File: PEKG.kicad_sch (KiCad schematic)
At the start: 115 parts, among them J1 AudioJack4, J2 AudioJack3_SwitchTR, U1 TLV9062, U12 NCS21802DMR2G, U13 NCS21802DMR2G, U2 TLV9062, U3 INA350CDSIDDFR, U7 TLV61070ADBVR, U8 NCS21802DMR2G

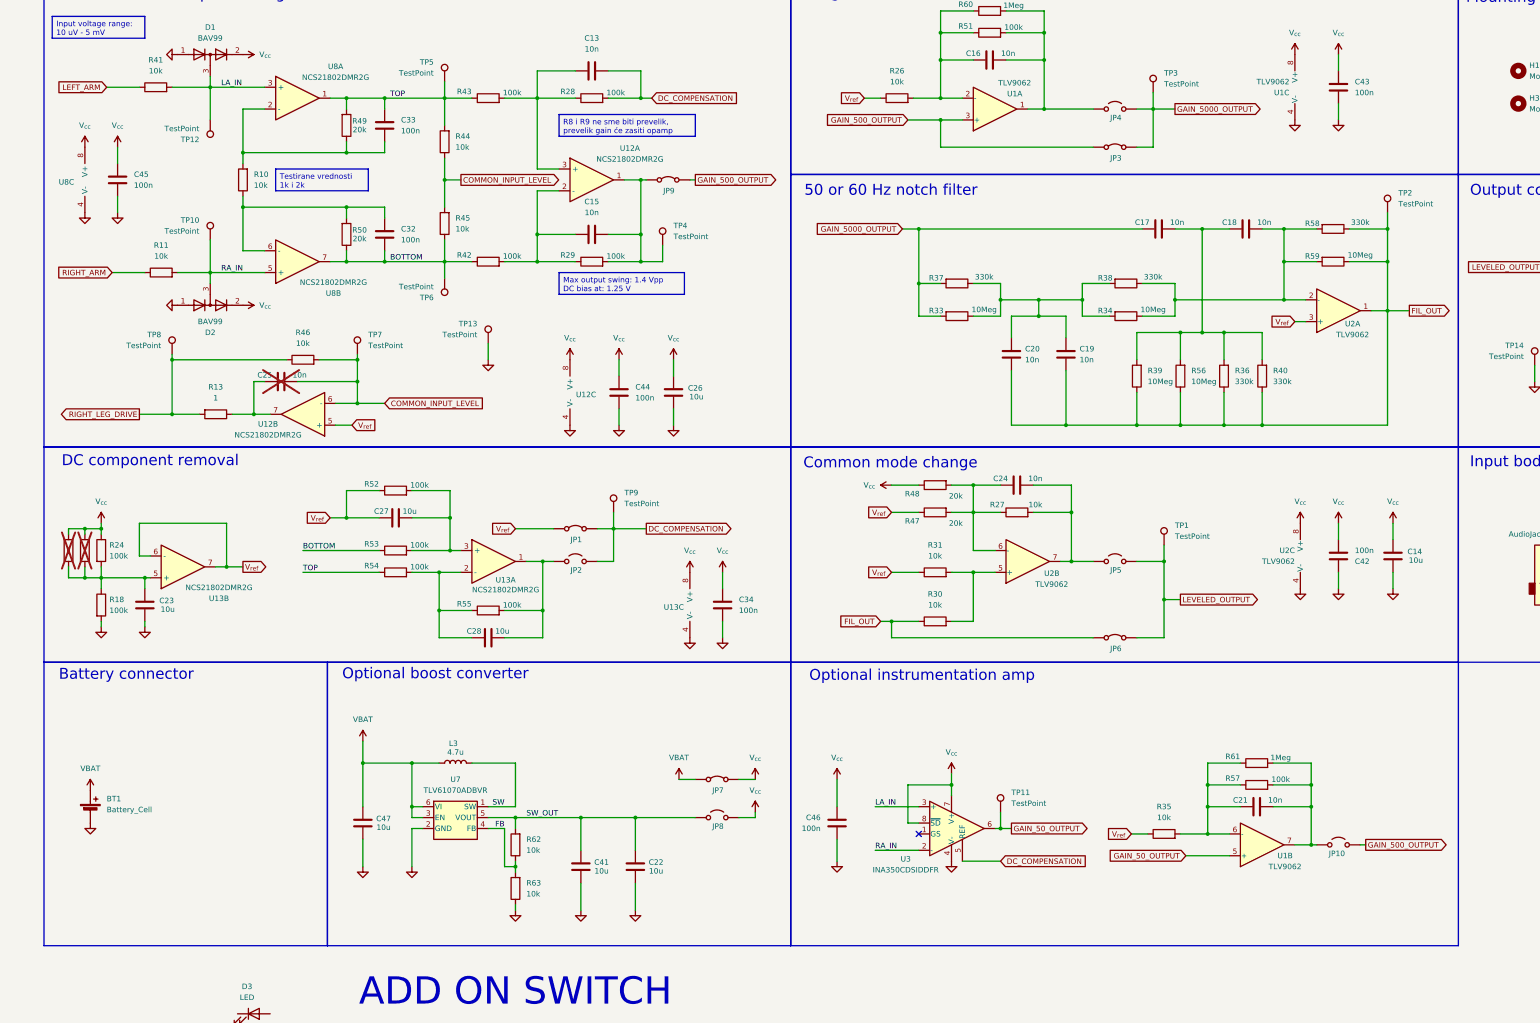
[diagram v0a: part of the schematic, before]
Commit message: added sw
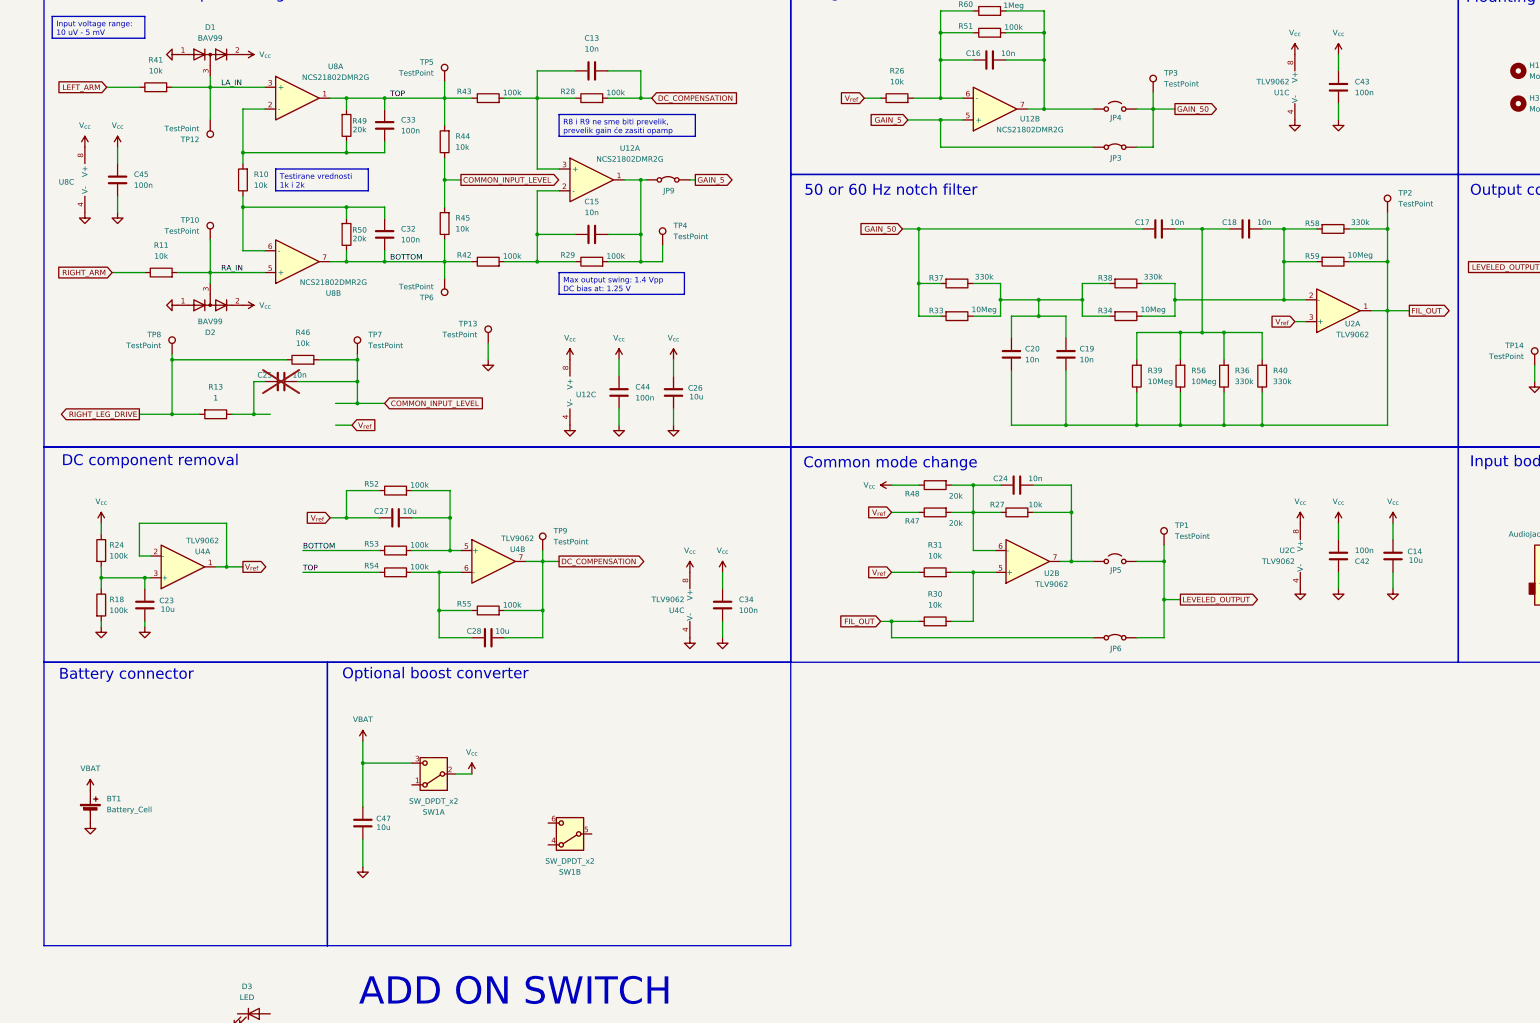
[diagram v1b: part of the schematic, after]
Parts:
- removed C21: 10n, Capacitor_SMD:C_0603_1608Metric_Pad1.08x0.95mm_HandSolder, symbol Device:C
- removed C22, C41: 10u, Capacitor_SMD:C_0603_1608Metric_Pad1.08x0.95mm_HandSolder, symbol Device:C
- removed C46: 100n, Capacitor_SMD:C_0603_1608Metric_Pad1.08x0.95mm_HandSolder, symbol Device:C
- removed JP1, JP7: Jumper_2_Bridged, Jumper:SolderJumper-2_P1.3mm_Bridged_RoundedPad1.0x1.5mm, symbol Jumper:Jumper_2_Bridged
- removed JP10, JP2, JP8: Jumper_2_Open, Jumper:SolderJumper-2_P1.3mm_Open_RoundedPad1.0x1.5mm, symbol Jumper:Jumper_2_Open
- removed L3: 4.7u, Inductor_SMD:L_Bourns_SRN6045TA, symbol Device:L
- removed R23, R32, R57: 100k, Resistor_SMD:R_0603_1608Metric_Pad0.98x0.95mm_HandSolder, symbol Device:R
- removed R35, R62, R63: 10k, Resistor_SMD:R_0603_1608Metric_Pad0.98x0.95mm_HandSolder, symbol Device:R
- removed R61: 1Meg, Resistor_SMD:R_0603_1608Metric_Pad0.98x0.95mm_HandSolder, symbol Device:R
- removed TP11: TestPoint, TestPoint:TestPoint_Pad_D3.0mm, symbol Connector:TestPoint
- removed unit 2 of U1
- removed unit 1 of U1
- removed U13: NCS21802DMR2G, Package_SO:OnSemi_Micro8, symbol voltmeter_lib:NCS21802DMR2G
- removed U3: INA350CDSIDDFR, Package_SO:MSOP-8_3x3mm_P0.65mm, symbol PEKG_lib:INA350CDSIDDFR
- removed U7: TLV61070ADBVR, Package_TO_SOT_SMD:SOT-23-6_Handsoldering, symbol DS100M08KV:TLV61070ADBVR
- added SW1: SW_DPDT_x2, PEKG:DPDT_bigger, symbol Switch:SW_DPDT_x2
- added U4: TLV9062, Package_SO:SOIC-8_3.9x4.9mm_P1.27mm, symbol Amplifier_Operational:TLV9062
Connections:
- net COMMON_INPUT_LEVEL: no longer U12.6 (-)
- net DC_COMPENSATION: now also C28.2, R55.2, U4.7
- net GND: now also U4.4 (V-)
- net VBAT: now also SW1.3 (C)
- net V_{cc}: now also SW1.2 (B), U4.8 (V+)
- net V_{ref}: now also U4.1, U4.2 (-); no longer U12.5 (+)
- net at C27.2, R52.2, R53.2: now also U4.5 (+)
- net at C23.1, R18.1, R24.2: now also U4.3 (+)
- net at C16.2, R26.2, R51.1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: now also U12.6 (-)
- net at C16.1, JP4.1 (A), R51.2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: now also U12.7
- net at C25.2, R13.1: no longer U12.7
- net at C28.1, R54.2, R55.1: now also U4.6 (-)
- net GAIN_5000_OUTPUT renamed GAIN_50
- net GAIN_500_OUTPUT renamed GAIN_5
- net GAIN_5: now also U12.5 (+)
- no-connect marks 5 -> 4
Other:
- note removed: "Optional instrumentation amp"
- moved on the sheet: TP9

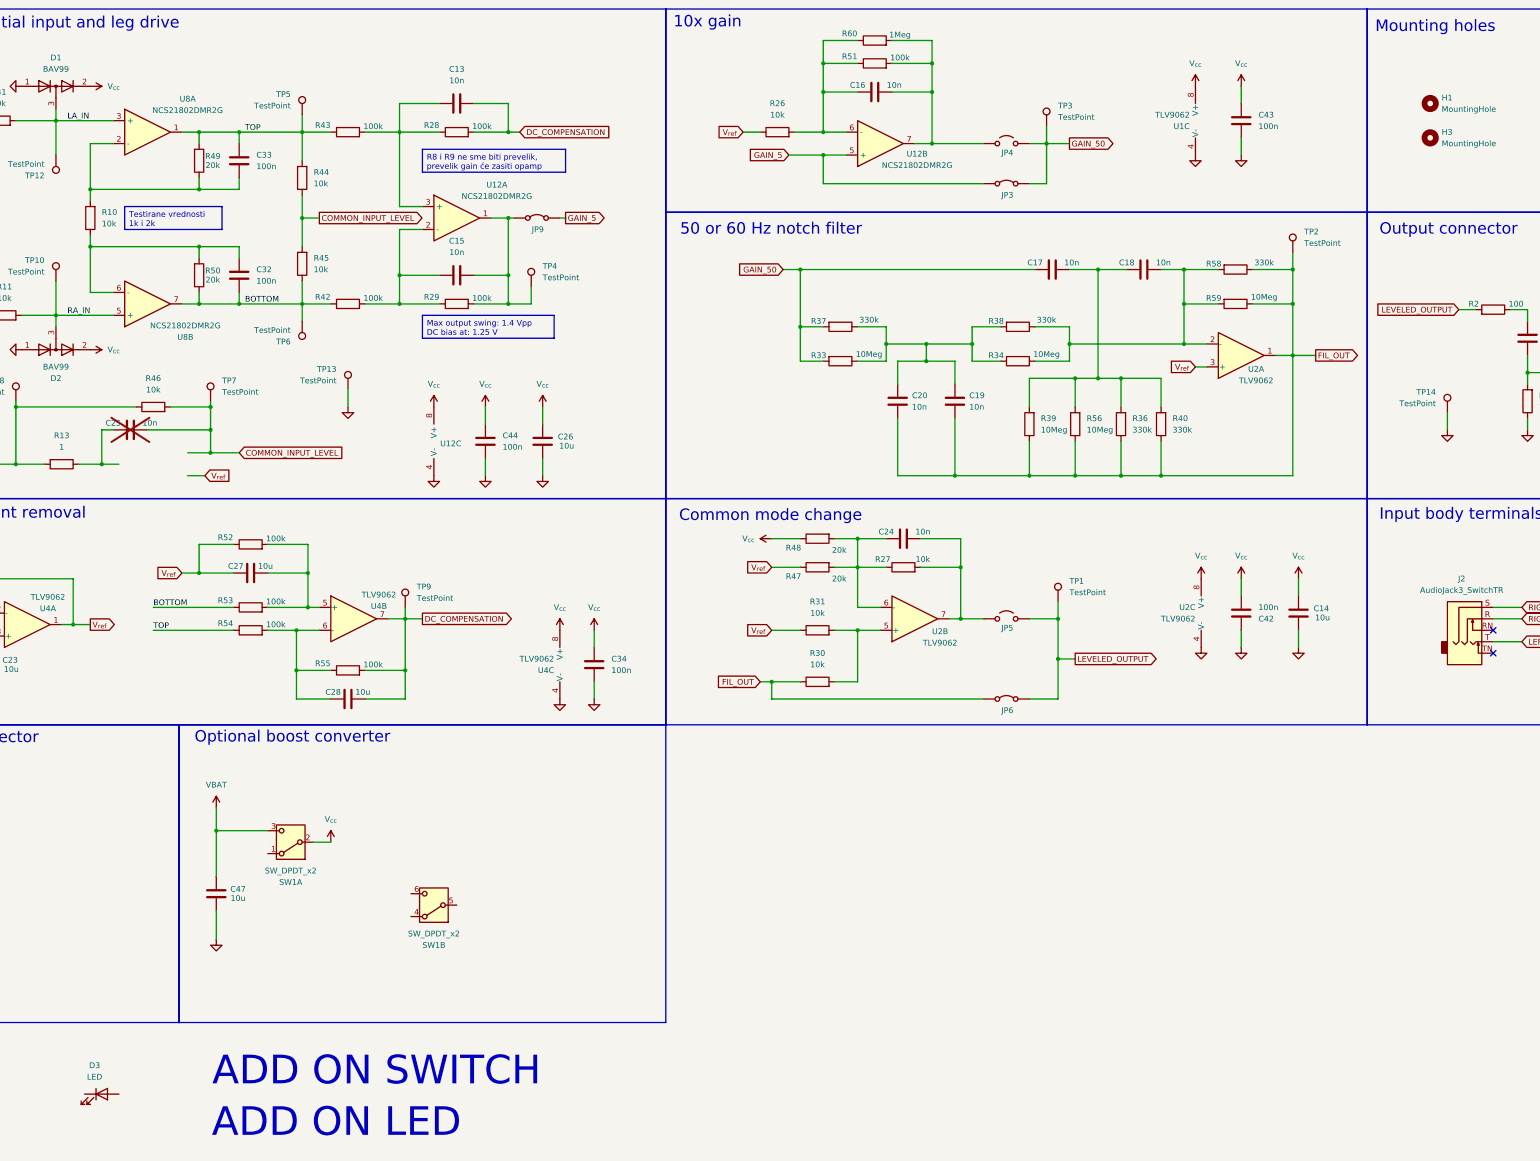
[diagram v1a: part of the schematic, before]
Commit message: opop
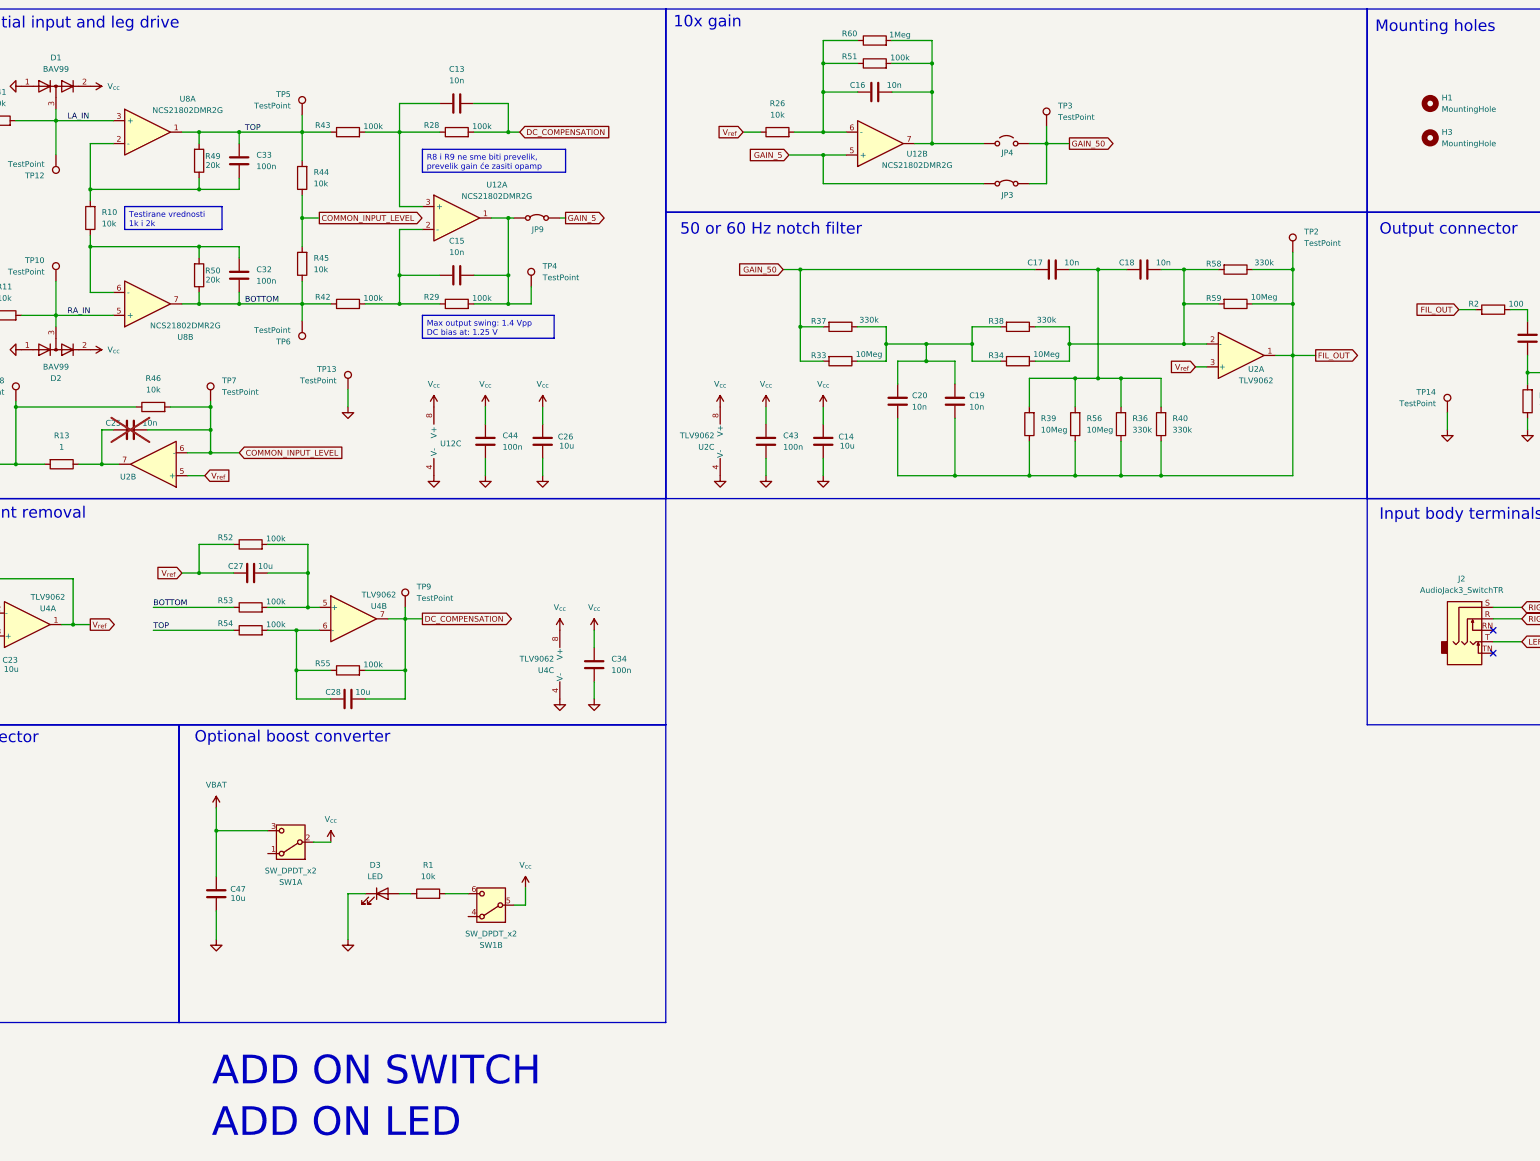
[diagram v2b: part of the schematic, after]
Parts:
- removed C24: 10n, Capacitor_SMD:C_0603_1608Metric_Pad1.08x0.95mm_HandSolder, symbol Device:C
- removed C42: 100n, Capacitor_SMD:C_0603_1608Metric_Pad1.08x0.95mm_HandSolder, symbol Device:C
- removed JP5: Jumper_2_Open, Jumper:SolderJumper-2_P1.3mm_Open_RoundedPad1.0x1.5mm, symbol Jumper:Jumper_2_Open
- removed JP6: Jumper_2_Bridged, Jumper:SolderJumper-2_P1.3mm_Bridged_RoundedPad1.0x1.5mm, symbol Jumper:Jumper_2_Bridged
- removed R27, R30, R31: 10k, Resistor_SMD:R_0603_1608Metric_Pad0.98x0.95mm_HandSolder, symbol Device:R
- removed R47, R48: 20k, Resistor_SMD:R_0603_1608Metric_Pad0.98x0.95mm_HandSolder, symbol Device:R
- removed TP1: TestPoint, TestPoint:TestPoint_Pad_D3.0mm, symbol Connector:TestPoint
- removed unit 3 of U2
- added R1: 10k, Resistor_SMD:R_0603_1608Metric_Pad0.98x0.95mm_HandSolder, symbol Device:R
- renumbered U1 to U2
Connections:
- net LEVELED_OUTPUT is gone; now on net FIL_OUT: R2.2
- net COMMON_INPUT_LEVEL: now also U2.6 (-)
- net GND: now also D3.1 (K)
- net V_{cc}: now also SW1.5 (B)
- net V_{ref}: now also U2.5 (+)
- net at U2.7: now also C25.2, R13.1
- net at D3.2 (A): now also R1.1
- net at SW1.6 (C): now also R1.2
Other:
- note removed: "Common mode change"
- moved on the sheet: C14, C43, D3, SW1B, U2B, U2C
